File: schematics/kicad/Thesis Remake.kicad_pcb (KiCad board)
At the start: 2 copper layers, 73 x 73 mm, 99 parts, among them J1 SJ2-35853B-SMT-TR, J2 Conn_01x18, J3 Conn_01x18, J4 Conn_01x01_Pin, J5 Conn_01x01_Pin, J6 Conn_01x01_Pin, J7 Conn_01x01_Pin, Q1 MMBT7002K, U10 MCP6001-OT, U11 MCP6001-OT, U2 PCM5102, U3 SN74LVC1G3157, U5 RT9080-33GJ5, U6 LM2940CT-5.0_MOD, U7 TPA711, U8 LM2940CT-5.0_MOD, U9 MCP6001-OT

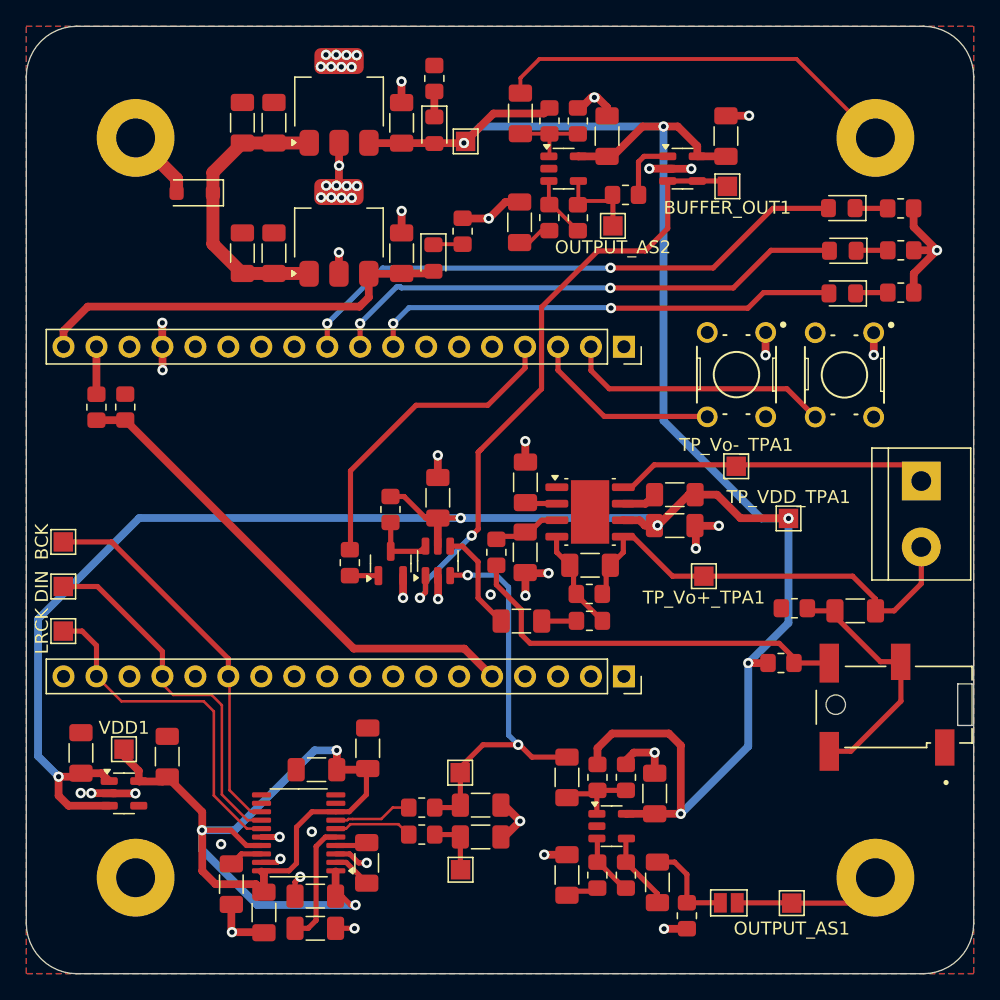
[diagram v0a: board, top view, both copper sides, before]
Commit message: code commits
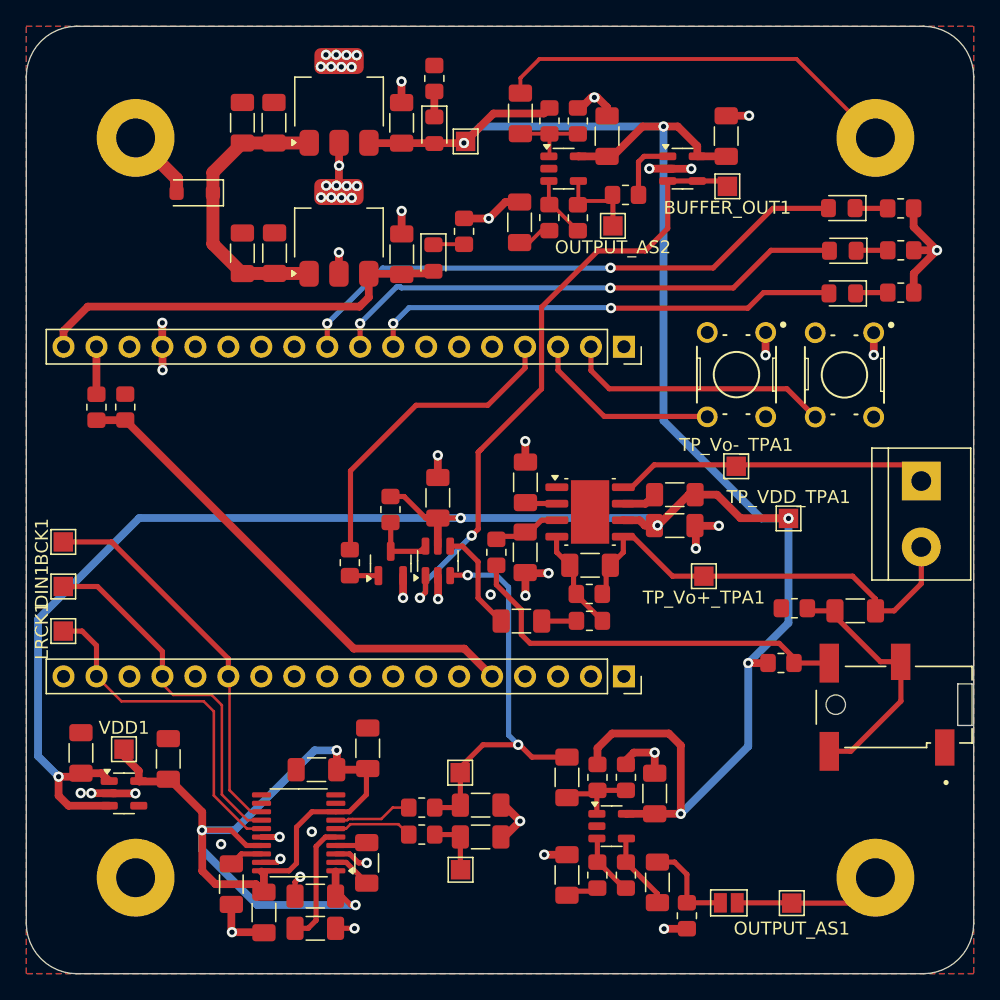
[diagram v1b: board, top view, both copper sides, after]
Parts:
- removed C_COUPLING_AMPSTAGE4: 10nF, Capacitor_SMD:C_1206_3216Metric_Pad1.33x1.80mm_HandSolder
- removed C_INPUT_LDO2: 0.47uF, Capacitor_SMD:C_1206_3216Metric_Pad1.33x1.80mm_HandSolder
- removed C_INPUT_RT1, C_OUTPUT_LDO2: 22uF, Capacitor_SMD:C_1206_3216Metric_Pad1.33x1.80mm_HandSolder
- removed C_IN_+15V_2: 10uF, Capacitor_SMD:C_1206_3216Metric_Pad1.33x1.80mm_HandSolder
- removed STATUS_LED2: 330, Resistor_SMD:R_0805_2012Metric_Pad1.20x1.40mm_HandSolder
- added C23: 10nF, Capacitor_SMD:C_1206_3216Metric_Pad1.33x1.80mm_HandSolder, F.Cu at (253.9, 38.5)
- added C4: 10uF, Capacitor_SMD:C_1206_3216Metric_Pad1.33x1.80mm_HandSolder, F.Cu at (216.7, 47.5)
- added C5: 0.47uF, Capacitor_SMD:C_1206_3216Metric_Pad1.33x1.80mm_HandSolder, F.Cu at (219.1, 47.5)
- added C6: 22uF, Capacitor_SMD:C_1206_3216Metric_Pad1.33x1.80mm_HandSolder, F.Cu at (228.9, 47.6)
- added C8: 22uF, Capacitor_SMD:C_1206_3216Metric_Pad1.33x1.80mm_HandSolder, F.Cu at (210.9, 86.5)
- added R2: 330, Resistor_SMD:R_0805_2012Metric_Pad1.20x1.40mm_HandSolder, F.Cu at (233.7, 45.8)
- renumbered BCK to BCK1, C_IN_+15V_3 to C1, CG2_PCM5102 to C10, C1_APS_PCM5102 to C11, C2_APS_PCM5102 to C12, C1_CPPS_PCM1 to C13, C2_CPPS_PCM1 to C14, C1_DPS_PCM1 to C15, C2_DPS_PCM1 to C16, C_GND_AMPSTAGE3 to C17, C_COUPLING_AMPSTAGE2 to C18, C_COUPLING_AMPSTAGE1 to C19, C_INPUT_LDO3 to C2, C_GND_AMPSTAGE1 to C20, C_IN_AMPSTAGE1 to C21, C_COUPLING_AMPSTAGE3 to C22, C_GND_AMPSTAGE2 to C24, CB_TPA1 to C25, C_SE/BTL_TPA1 to C26, C_INPUT_TPA1 to C27, C_INPUT_TPA2 to C28, CF_TPA711 to C29, C_OUTPUT_LDO3 to C3, C_INPUT_TPA3 to C30, C_COUPLING_MUX2 to C31, CA_PCM5102 to C32, CI_TPA711 to C33, C_INPUT_RT9080 to C7, CG1_PCM5102 to C9, DIN to DIN1, LRCK to LRCK1, STATUS_LED3 to R1, R3 to R10, R4 to R11, RG2 to R12, RF2 to R13, R13 to R14, R12 to R15, RF_TPA711 to R16, RI_TPA711 to R17, R11 to R18, RL1 to R19, RG3 to R20, R_LADDER_2 to R21, R_LADDER_3 to R22, R5 to R23, R6 to R24, R7 to R25, ROUTDACL1 to R3, ROUTDACR1 to R4, R1 to R5, R2 to R6, RG1 to R7, RF1 to R8, R_COUPLING_AMPSTAGE1 to R9
